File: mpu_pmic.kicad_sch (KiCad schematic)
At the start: 48 parts, among them U501 STPMIC1DPQR

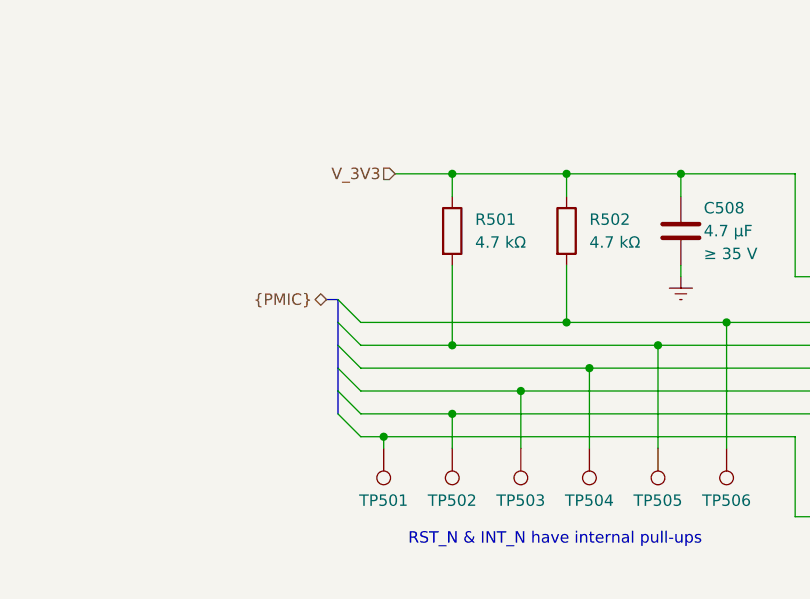
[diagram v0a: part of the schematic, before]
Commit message: Add a debug section
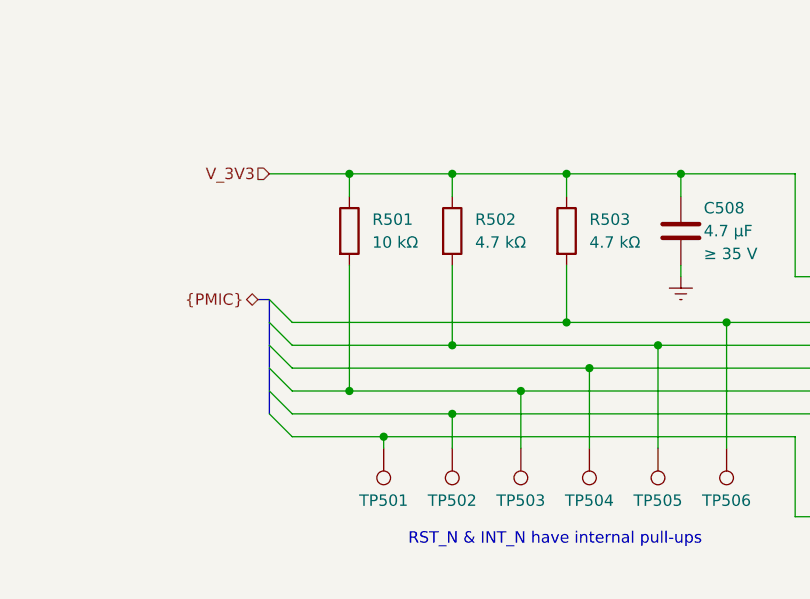
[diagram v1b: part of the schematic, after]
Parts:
- added R501: 10 kΩ, perfect_footprints:R_0402_1005Metric, symbol Device:R
- renumbered R501 to R502, R502 to R503
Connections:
- net RST_N: now also R501.2
- net V_3V3: now also R501.1
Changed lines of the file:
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@@
 	)
 	(junction
+		(at 97.79 200.66)
+		(diameter 0)
+		(color 0 0 0 0)
+	)
+	(junction
 		(at 349.25 152.4)
 		(diameter 0)
@@
 	)
 	(junction
+		(at 97.79 176.53)
+		(diameter 0)
+		(color 0 0 0 0)
+	)
+	(junction
 		(at 142.24 149.86)
 		(diameter 0)
@@
 	)
 	(bus_entry
-		(at 99.06 203.2)
+		(at 91.44 203.2)
 		(size -2.54 -2.54)
 		(stroke
@@
 	)
 	(bus_entry
-		(at 99.06 195.58)
+		(at 91.44 195.58)
 		(size -2.54 -2.54)
 		(stroke
@@
 	)
 	(bus_entry
-		(at 99.06 205.74)
+		(at 91.44 205.74)
 		(size -2.54 -2.54)
 		(stroke
@@
 	)
 	(bus_entry
-		(at 99.06 193.04)
+		(at 91.44 193.04)
 		(size -2.54 -2.54)
 		(stroke
@@
 	)
 	(bus_entry
-		(at 99.06 200.66)
+		(at 91.44 200.66)
 		(size -2.54 -2.54)
 		(stroke
@@
 	)
 	(bus_entry
-		(at 99.06 198.12)
+		(at 91.44 198.12)
 		(size -2.54 -2.54)
 		(stroke
@@
 	(wire
 		(pts
-			(xy 102.87 176.53) (xy 109.22 176.53)
+			(xy 88.9 176.53) (xy 97.79 176.53)
 		)
 		(stroke
@@
 	(wire
 		(pts
+			(xy 97.79 176.53) (xy 109.22 176.53)
+		)
+		(stroke
+			(width 0)
+			(type default)
+		)
+	)
+	(wire
+		(pts
 			(xy 116.84 125.73) (xy 104.14 125.73)
 		)
@@
 	(bus
 		(pts
-			(xy 95.25 190.5) (xy 96.52 190.5)
+			(xy 87.63 190.5) (xy 88.9 190.5)
 		)
 		(stroke
@@
 	(wire
 		(pts
-			(xy 99.06 198.12) (xy 124.46 198.12)
+			(xy 91.44 198.12) (xy 124.46 198.12)
 		)
 		(stroke
@@
 	(wire
 		(pts
-			(xy 99.06 195.58) (xy 109.22 195.58)
+			(xy 91.44 195.58) (xy 109.22 195.58)
 		)
 		(stroke
@@
 	(wire
 		(pts
+			(xy 97.79 176.53) (xy 97.79 179.07)
+		)
+		(stroke
+			(width 0)
+			(type default)
+		)
+	)
+	(wire
+		(pts
 			(xy 109.22 176.53) (xy 121.92 176.53)
 		)
@@
 	(wire
 		(pts
-			(xy 99.06 205.74) (xy 101.6 205.74)
+			(xy 91.44 205.74) (xy 101.6 205.74)
 		)
 		(stroke
@@
 	(bus
 		(pts
-			(xy 96.52 198.12) (xy 96.52 195.58)
+			(xy 88.9 198.12) (xy 88.9 195.58)
 		)
 		(stroke
@@
 	(bus
 		(pts
-			(xy 96.52 200.66) (xy 96.52 198.12)
+			(xy 88.9 200.66) (xy 88.9 198.12)
 		)
 		(stroke
@@
 	(bus
 		(pts
-			(xy 96.52 193.04) (xy 96.52 195.58)
+			(xy 88.9 193.04) (xy 88.9 195.58)
 		)
 		(stroke
@@
 	(wire
 		(pts
-			(xy 99.06 200.66) (xy 116.84 200.66)
+			(xy 91.44 200.66) (xy 97.79 200.66)
 		)
 		(stroke
@@
 	(bus
 		(pts
-			(xy 96.52 203.2) (xy 96.52 200.66)
+			(xy 88.9 203.2) (xy 88.9 200.66)
 		)
 		(stroke
@@
 	(bus
 		(pts
-			(xy 96.52 193.04) (xy 96.52 190.5)
+			(xy 88.9 193.04) (xy 88.9 190.5)
 		)
 		(stroke
@@
 	(wire
 		(pts
-			(xy 99.06 203.2) (xy 109.22 203.2)
+			(xy 91.44 203.2) (xy 109.22 203.2)
 		)
 		(stroke
@@
 	(wire
 		(pts
-			(xy 99.06 193.04) (xy 121.92 193.04)
+			(xy 91.44 193.04) (xy 121.92 193.04)
 		)
 		(stroke
@@
 	(wire
 		(pts
+			(xy 97.79 200.66) (xy 116.84 200.66)
+		)
+		(stroke
+			(width 0)
+			(type default)
+		)
+	)
+	(wire
+		(pts
 			(xy 336.55 240.03) (xy 339.09 240.03)
 		)
@@
 	(wire
 		(pts
+			(xy 97.79 186.69) (xy 97.79 200.66)
+		)
+		(stroke
+			(width 0)
+			(type default)
+		)
+	)
+	(wire
+		(pts
 			(xy 302.26 166.37) (xy 302.26 165.1)
 		)
@@
 	(hierarchical_label "V_3V3"
 		(shape input)
-		(at 102.87 176.53 180)
+		(at 88.9 176.53 180)
 		(effects
 			(font
@@
 	(hierarchical_label "{PMIC}"
 		(shape bidirectional)
-		(at 95.25 190.5 180)
+		(at 87.63 190.5 180)
 		(effects
 			(font
@@
 		(on_board yes)
 		(dnp no)
-		(property "Reference" "R502"
+		(property "Reference" "R503"
 			(at 124.46 181.6099 0)
 			(effects
@@
 			(project "linux-sbc"
 				(path "/fa11a02f-8043-4153-ab69-88d766503017/2d01087b-54dc-4f43-9cc7-a0ba17201776/8c2fc621-bdce-4f4c-8cac-9098b808a2b8"
-					(reference "R502")
+					(reference "R503")
 					(unit 1)
 				)
@@
 	)
 	(symbol
+		(lib_id "Device:R")
+		(at 97.79 182.88 0)
+		(unit 1)
+		(exclude_from_sim no)
+		(in_bom yes)
+		(on_board yes)
+		(dnp no)
+		(property "Reference" "R501"
+			(at 100.33 181.6099 0)
+			(effects
+				(font
+					(size 1.27 1.27)
+				)
+				(justify left)
+			)
+		)
+		(property "Value" "10 kΩ"
+			(at 100.33 184.1499 0)
+			(effects
+				(font
+					(size 1.27 1.27)
+				)
+				(justify left)
+			)
+		)
+		(property "Footprint" "perfect_footprints:R_0402_1005Metric"
+			(at 96.012 182.88 90)
+			(effects
+				(font
+					(size 1.27 1.27)
+				)
+				(hide yes)
+			)
+		)
+		(property "Datasheet" "https://www.we-online.com/components/products/datasheet/560112110020.pdf"
+			(at 97.79 182.88 0)
+			(effects
+				(font
+					(size 1.27 1.27)
+				)
+				(hide yes)
+			)
+		)
+		(property "Description" "Resistor"
+			(at 97.79 182.88 0)
+			(effects
+				(font
+					(size 1.27 1.27)
+				)
+				(hide yes)
+			)
+		)
+		(property "DigiKey Part Number" "732-560112110020CT-ND"
+			(at 97.79 182.88 0)
+			(effects
+				(font
+					(size 1.27 1.27)
+				)
+				(hide yes)
+			)
+		)
+		(property "MPN" "560112110020"
+			(at 97.79 182.88 0)
+			(effects
+				(font
+					(size 1.27 1.27)
+				)
+				(hide yes)
+			)
+		)
+		(property "Manufacturer" "Würth Elektronik"
+			(at 97.79 182.88 0)
+			(effects
+				(font
+					(size 1.27 1.27)
+				)
+				(hide yes)
+			)
+		)
+		(property "Temperature Coefficient" ""
+			(at 97.79 182.88 0)
+			(effects
+				(font
+					(size 1.27 1.27)
+				)
+				(hide yes)
+			)
+		)
+		(pin "2"
+		)
+		(pin "1"
+		)
+		(instances
+			(project "linux-sbc"
+				(path "/fa11a02f-8043-4153-ab69-88d766503017/2d01087b-54dc-4f43-9cc7-a0ba17201776/8c2fc621-bdce-4f4c-8cac-9098b808a2b8"
+					(reference "R501")
+					(unit 1)
+				)
+			)
+		)
+	)
+	(symbol
 		(lib_id "STMicroelectronics:STPMIC1DPQR")
 		(at 182.88 160.02 0)
@@
 		(on_board yes)
 		(dnp no)
-		(property "Reference" "R501"
+		(property "Reference" "R502"
 			(at 111.76 181.6099 0)
 			(effects
@@
 			(project "linux-sbc"
 				(path "/fa11a02f-8043-4153-ab69-88d766503017/2d01087b-54dc-4f43-9cc7-a0ba17201776/8c2fc621-bdce-4f4c-8cac-9098b808a2b8"
-					(reference "R501")
+					(reference "R502")
 					(unit 1)
 				)
